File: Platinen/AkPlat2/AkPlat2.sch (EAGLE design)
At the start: 26 parts, among them M1 22-23-2021, M2 22-23-2021, M3 22-23-2021, M4 22-23-2021, X2 332-02, X3 332-02

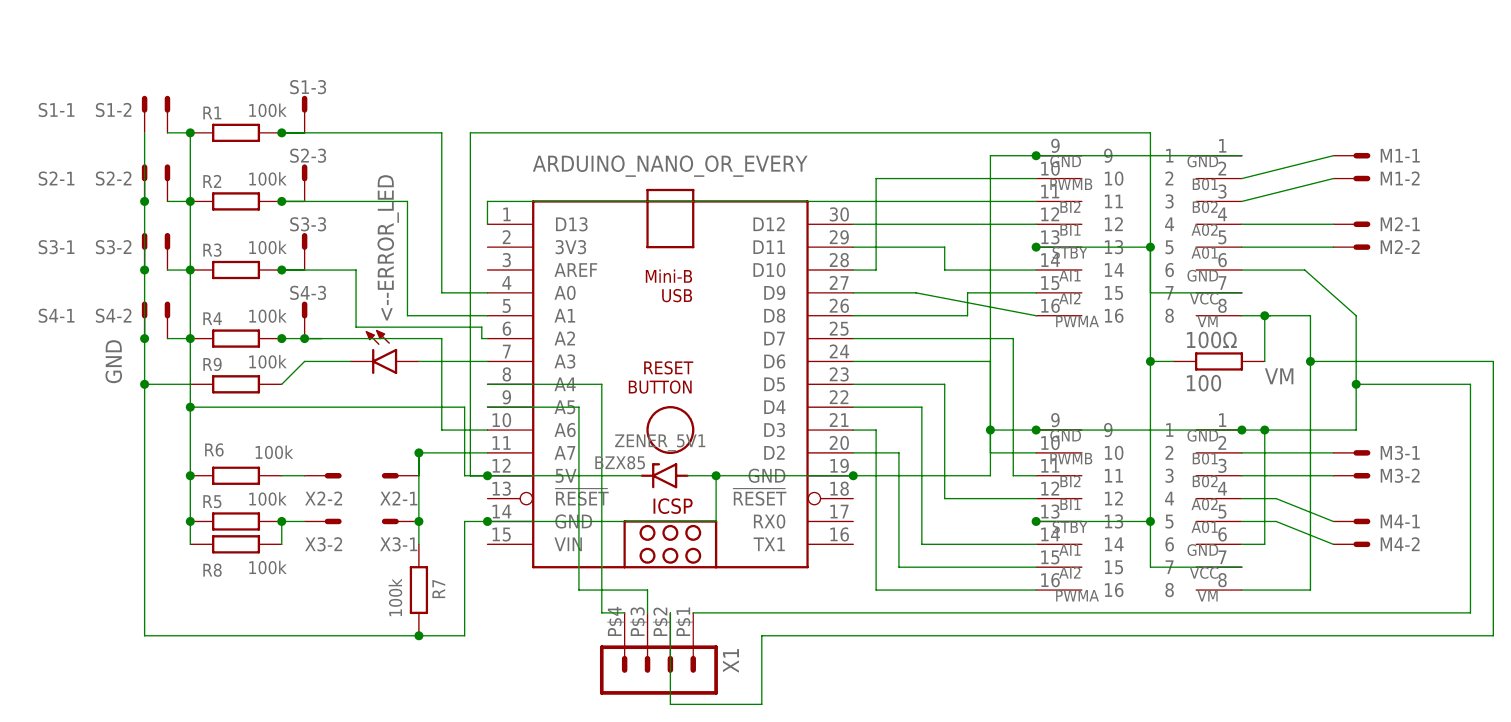
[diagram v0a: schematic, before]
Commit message: reverted changes
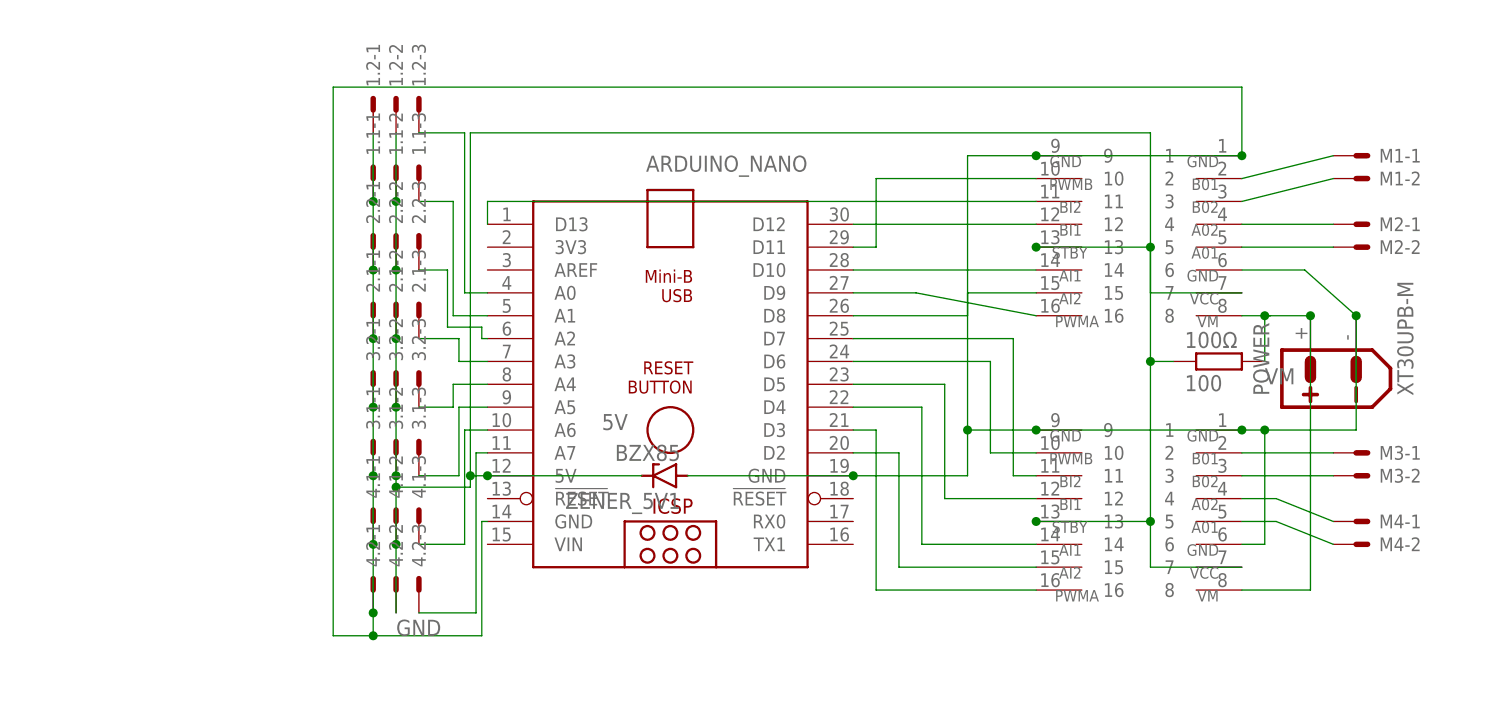
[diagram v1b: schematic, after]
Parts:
- removed <--ERROR_LED: (no value), led:LED3MM
- removed R1, R2, R3, R4, R5, R6, R7, R8, R9: 100k, rcl:R-EU_R0402
- removed S1, S2, S3, S4: 22-23-2031, con-molex:22-23-2031
- removed X1: (no value), con-molex-micro-fit-3_0:HEADER_POS4_43045-0412
- removed X2, X3: 332-02, con-garry:332-02
- added 1.1, 1.2, 2.1, 2.2, 3.1, 3.2, 4.1, 4.2: 22-23-2031, con-molex:22-23-2031
- added POWER: XT30UPB-M, amass:XT30UPB-M
- renumbered ARDUINO_NANO_OR_EVERY to ARDUINO_NANO
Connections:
- removed net N$1: ARDUINO_NANO.A4, X1.4
- removed net N$15: R6.1, X2-2.S
- removed net N$2: ARDUINO_NANO.A5, X1.3
- removed net N$24: R5.2, R8.2, X3-2.S
- removed net N$25: <--ERROR_LED.A, ARDUINO_NANO.A3
- removed net N$8: ARDUINO_NANO.A7, R7.1, X2-1.S, X3-1.S
- new net N$27: 4.1-3.S, ARDUINO_NANO.A6
- new net N$30: 3.1-3.S, ARDUINO_NANO.A5
- new net N$31: 3.2-3.S, ARDUINO_NANO.A4
- net 5V: now also 1.1-2.S, 1.2-2.S, 2.1-2.S, 2.2-2.S, 3.1-2.S, 3.2-2.S, 4.1-2.S, 4.2-2.S; no longer R1.1, R2.1, R3.1, R4.1, R5.1, R6.2, R8.1, S1-2.S, S2-2.S, S3-2.S, S4-2.S
- net GND: now also 1.1-1.S, 1.2-1.S, 2.1-1.S, 2.2-1.S, 3.1-1.S, 3.2-1.S, 4.1-1.S, 4.2-1.S, POWER.-; no longer R7.2, R9.1, S1-1.S, S2-1.S, S3-1.S, S4-1.S, X1.1
- net N$26: now also 4.2-3.S, ARDUINO_NANO.A7; no longer <--ERROR_LED.C, R9.2
- net N$32: now also 2.1-3.S, ARDUINO_NANO.A3; no longer ARDUINO_NANO.A6, R4.2, S4-3.S
- net N$33: now also 2.2-3.S; no longer R3.2, S3-3.S
- net N$34: now also 1.1-3.S; no longer R2.2, S2-3.S
- net N$35: now also 1.2-3.S; no longer R1.2, S1-3.S
- net N$6: now also ARDUINO_NANO.D11; no longer ARDUINO_NANO.D10
- net N$7: now also ARDUINO_NANO.D10; no longer ARDUINO_NANO.D11
- net VM: now also POWER.+; no longer X1.2

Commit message: improvisation, code in CODE_HERE.py
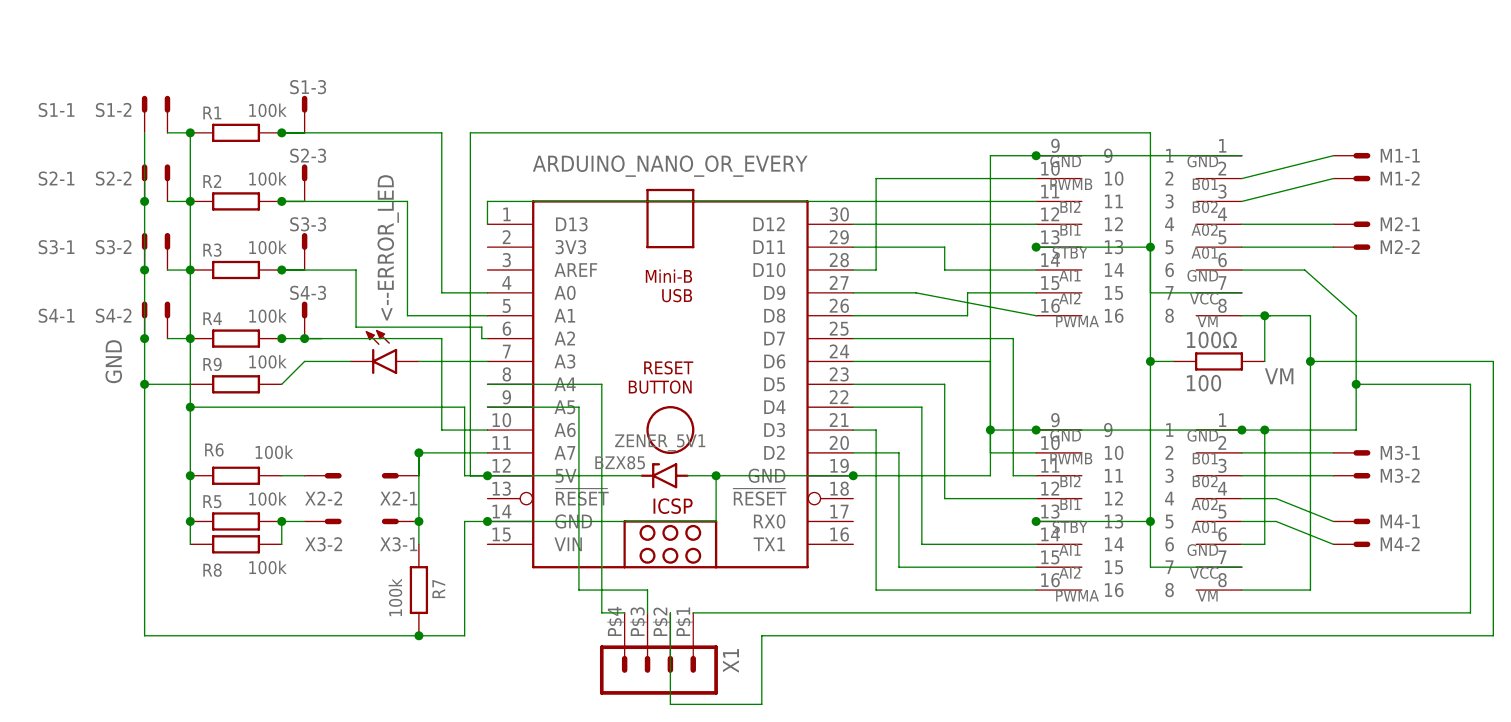
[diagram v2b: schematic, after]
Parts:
- removed 1.1, 1.2, 2.1, 2.2, 3.1, 3.2, 4.1, 4.2: 22-23-2031, con-molex:22-23-2031
- removed POWER: XT30UPB-M, amass:XT30UPB-M
- added <--ERROR_LED: (no value), led:LED3MM
- added R1, R2, R3, R4, R5, R6, R7, R8, R9: 100k, rcl:R-EU_R0402
- added S1, S2, S3, S4: 22-23-2031, con-molex:22-23-2031
- added X1: (no value), con-molex-micro-fit-3_0:HEADER_POS4_43045-0412
- added X2, X3: 332-02, con-garry:332-02
- renumbered ARDUINO_NANO to ARDUINO_NANO_OR_EVERY
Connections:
- removed net N$27: 4.1-3.S, ARDUINO_NANO_OR_EVERY.A6
- removed net N$30: 3.1-3.S, ARDUINO_NANO_OR_EVERY.A5
- removed net N$31: 3.2-3.S, ARDUINO_NANO_OR_EVERY.A4
- new net N$1: ARDUINO_NANO_OR_EVERY.A4, X1.4
- new net N$15: R6.1, X2-2.S
- new net N$2: ARDUINO_NANO_OR_EVERY.A5, X1.3
- new net N$24: R5.2, R8.2, X3-2.S
- new net N$25: <--ERROR_LED.A, ARDUINO_NANO_OR_EVERY.A3
- new net N$8: ARDUINO_NANO_OR_EVERY.A7, R7.1, X2-1.S, X3-1.S
- net 5V: now also R1.1, R2.1, R3.1, R4.1, R5.1, R6.2, R8.1, S1-2.S, S2-2.S, S3-2.S, S4-2.S; no longer 1.1-2.S, 1.2-2.S, 2.1-2.S, 2.2-2.S, 3.1-2.S, 3.2-2.S, 4.1-2.S, 4.2-2.S
- net GND: now also R7.2, R9.1, S1-1.S, S2-1.S, S3-1.S, S4-1.S, X1.1; no longer 1.1-1.S, 1.2-1.S, 2.1-1.S, 2.2-1.S, 3.1-1.S, 3.2-1.S, 4.1-1.S, 4.2-1.S, POWER.-
- net N$26: now also <--ERROR_LED.C, R9.2; no longer 4.2-3.S, ARDUINO_NANO_OR_EVERY.A7
- net N$32: now also ARDUINO_NANO_OR_EVERY.A6, R4.2, S4-3.S; no longer 2.1-3.S, ARDUINO_NANO_OR_EVERY.A3
- net N$33: now also R3.2, S3-3.S; no longer 2.2-3.S
- net N$34: now also R2.2, S2-3.S; no longer 1.1-3.S
- net N$35: now also R1.2, S1-3.S; no longer 1.2-3.S
- net N$6: now also ARDUINO_NANO_OR_EVERY.D10; no longer ARDUINO_NANO_OR_EVERY.D11
- net N$7: now also ARDUINO_NANO_OR_EVERY.D11; no longer ARDUINO_NANO_OR_EVERY.D10
- net VM: now also X1.2; no longer POWER.+
